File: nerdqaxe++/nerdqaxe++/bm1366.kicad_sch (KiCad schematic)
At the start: 82 parts, among them U19 BM1370_mode1, U20 BM1370, U25 BM1370_mode1, U26 BM1370_mode1, U6 SN74AVC4T774, U8 25MHz

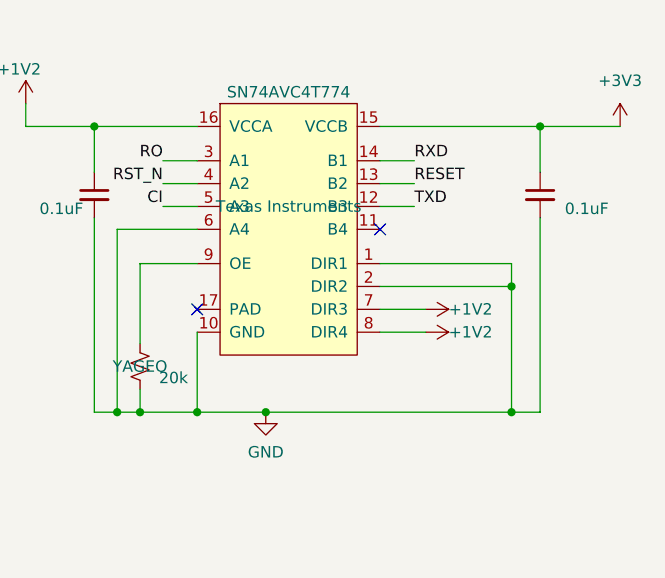
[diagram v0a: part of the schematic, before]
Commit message: Rev. 6.1
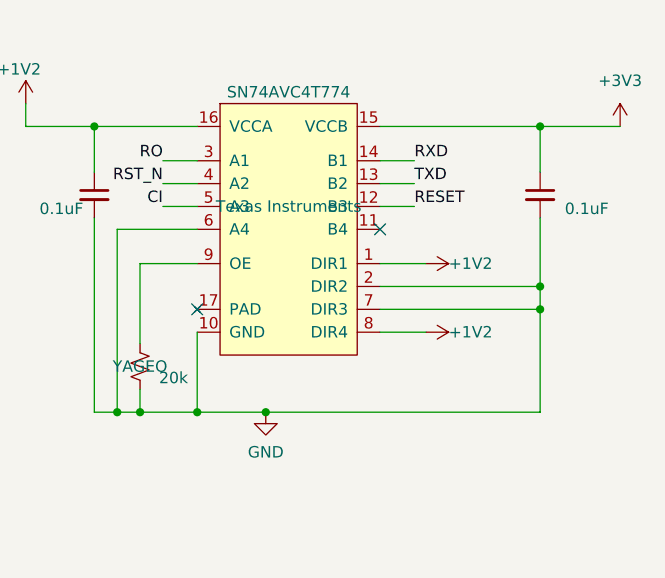
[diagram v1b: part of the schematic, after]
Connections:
- net +1V2: now also U6.1 (DIR1); no longer U6.7 (DIR3)
- net GND: now also U6.7 (DIR3); no longer U6.1 (DIR1)
- net RESET: now also U6.12 (B3); no longer U6.13 (B2)
- net TXD: now also U6.13 (B2); no longer U6.12 (B3)
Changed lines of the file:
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@@
 	)
 	(junction
-		(at 376.555 157.48)
-		(diameter 0)
-		(color 0 0 0 0)
-	)
-	(junction
 		(at 209.55 257.81)
 		(diameter 0)
@@
 	)
 	(junction
-		(at 198.12 233.68)
+		(at 379.73 143.51)
 		(diameter 0)
 		(color 0 0 0 0)
 	)
 	(junction
-		(at 200.66 229.87)
+		(at 198.12 233.68)
 		(diameter 0)
 		(color 0 0 0 0)
 	)
 	(junction
-		(at 196.85 257.81)
+		(at 200.66 229.87)
 		(diameter 0)
 		(color 0 0 0 0)
 	)
 	(junction
-		(at 376.555 143.51)
+		(at 196.85 257.81)
 		(diameter 0)
 		(color 0 0 0 0)
@@
 	)
 	(junction
+		(at 379.73 146.05)
+		(diameter 0)
+		(color 0 0 0 0)
+	)
+	(junction
 		(at 156.21 81.28)
 		(diameter 0)
@@
 	(wire
 		(pts
-			(xy 361.95 140.97) (xy 376.555 140.97)
-		)
-		(stroke
-			(width 0)
-			(type default)
-		)
-	)
-	(wire
-		(pts
 			(xy 151.13 127) (xy 156.21 127)
 		)
@@
 	(wire
 		(pts
-			(xy 376.555 140.97) (xy 376.555 143.51)
-		)
-		(stroke
-			(width 0)
-			(type default)
-		)
-	)
-	(wire
-		(pts
 			(xy 220.98 250.19) (xy 220.98 248.92)
 		)
@@
 	(wire
 		(pts
-			(xy 376.555 143.51) (xy 376.555 157.48)
-		)
-		(stroke
-			(width 0)
-			(type default)
-		)
-	)
-	(wire
-		(pts
 			(xy 179.07 55.88) (xy 179.07 41.91)
 		)
@@
 	(wire
 		(pts
+			(xy 349.25 157.48) (xy 379.73 157.48)
+		)
+		(stroke
+			(width 0)
+			(type default)
+		)
+	)
+	(wire
+		(pts
 			(xy 262.89 81.28) (xy 262.89 83.82)
 		)
@@
 	(wire
 		(pts
-			(xy 361.95 146.05) (xy 367.03 146.05)
-		)
-		(stroke
-			(width 0)
-			(type default)
-		)
-	)
-	(wire
-		(pts
 			(xy 118.11 161.29) (xy 102.87 161.29)
 		)
@@
 	(wire
 		(pts
-			(xy 361.95 143.51) (xy 376.555 143.51)
-		)
-		(stroke
-			(width 0)
-			(type default)
-		)
-	)
-	(wire
-		(pts
 			(xy 29.21 31.75) (xy 38.1 31.75)
 		)
@@
 	(wire
 		(pts
+			(xy 361.95 143.51) (xy 379.73 143.51)
+		)
+		(stroke
+			(width 0)
+			(type default)
+		)
+	)
+	(wire
+		(pts
 			(xy 156.21 135.89) (xy 198.12 135.89)
 		)
@@
 	(wire
 		(pts
+			(xy 361.95 140.97) (xy 367.03 140.97)
+		)
+		(stroke
+			(width 0)
+			(type default)
+		)
+	)
+	(wire
+		(pts
 			(xy 187.96 255.27) (xy 187.96 257.81)
 		)
@@
 	(wire
 		(pts
+			(xy 379.73 146.05) (xy 379.73 157.48)
+		)
+		(stroke
+			(width 0)
+			(type default)
+		)
+	)
+	(wire
+		(pts
 			(xy 191.77 227.33) (xy 191.77 229.87)
 		)
@@
 	(wire
 		(pts
-			(xy 379.73 135.89) (xy 379.73 157.48)
+			(xy 379.73 135.89) (xy 379.73 143.51)
 		)
 		(stroke
@@
 	(wire
 		(pts
+			(xy 379.73 143.51) (xy 379.73 146.05)
+		)
+		(stroke
+			(width 0)
+			(type default)
+		)
+	)
+	(wire
+		(pts
 			(xy 167.64 53.34) (xy 199.39 53.34)
 		)
@@
 	(wire
 		(pts
-			(xy 349.25 157.48) (xy 376.555 157.48)
+			(xy 135.89 39.37) (xy 135.89 41.91)
 		)
 		(stroke
@@
 	(wire
 		(pts
-			(xy 135.89 39.37) (xy 135.89 41.91)
+			(xy 260.35 41.91) (xy 262.89 41.91)
 		)
 		(stroke
@@
 	(wire
 		(pts
-			(xy 260.35 41.91) (xy 262.89 41.91)
+			(xy 207.01 242.57) (xy 210.82 242.57)
 		)
 		(stroke
@@
 	(wire
 		(pts
-			(xy 207.01 242.57) (xy 210.82 242.57)
+			(xy 104.14 198.12) (xy 104.14 199.39)
 		)
 		(stroke
@@
 	(wire
 		(pts
-			(xy 104.14 198.12) (xy 104.14 199.39)
+			(xy 102.87 76.2) (xy 118.11 76.2)
 		)
 		(stroke
@@
 	(wire
 		(pts
-			(xy 102.87 76.2) (xy 118.11 76.2)
+			(xy 361.95 146.05) (xy 379.73 146.05)
 		)
 		(stroke
@@
 	(wire
 		(pts
-			(xy 376.555 157.48) (xy 379.73 157.48)
-		)
-		(stroke
-			(width 0)
-			(type default)
-		)
-	)
-	(wire
-		(pts
 			(xy 198.12 58.42) (xy 198.12 81.28)
 		)
@@
 		)
 	)
-	(label "RESET"
-		(at 365.76 132.08 0)
-		(effects
-			(font
-				(size 1.27 1.27)
-			)
-			(justify left bottom)
-		)
-	)
 	(label "CI"
 		(at 337.82 134.62 180)
@@
 		)
 	)
-	(label "TXD"
-		(at 365.76 134.62 0)
-		(effects
-			(font
-				(size 1.27 1.27)
-			)
-			(justify left bottom)
-		)
-	)
 	(label "RXD"
 		(at 365.76 129.54 0)
@@
 		)
 	)
+	(label "TXD"
+		(at 365.76 132.08 0)
+		(effects
+			(font
+				(size 1.27 1.27)
+			)
+			(justify left bottom)
+		)
+	)
 	(label "RST_N"
 		(at 101.6 60.96 0)
@@
 		)
 	)
+	(label "RESET"
+		(at 365.76 134.62 0)
+		(effects
+			(font
+				(size 1.27 1.27)
+			)
+			(justify left bottom)
+		)
+	)
 	(label "RO"
 		(at 337.82 129.54 180)
@@
 	(symbol
 		(lib_id "power:+1V2")
-		(at 367.03 146.05 270)
+		(at 367.03 140.97 270)
 		(unit 1)
 		(exclude_from_sim no)
@@
 		(dnp no)
 		(property "Reference" "#PWR0177"
-			(at 363.22 146.05 0)
+			(at 363.22 140.97 0)
 			(effects
 				(font
@@
 		)
 		(property "Value" "+1V2"
-			(at 369.57 146.05 90)
+			(at 369.57 140.97 90)
 			(effects
 				(font
@@
 		)
 		(property "Footprint" ""
-			(at 367.03 146.05 0)
+			(at 367.03 140.97 0)
 			(effects
 				(font
@@
 		)
 		(property "Datasheet" ""
-			(at 367.03 146.05 0)
+			(at 367.03 140.97 0)
 			(effects
 				(font
@@
 		)
 		(property "Description" "Power symbol creates a global label with name \"+1V2\""
-			(at 367.03 146.05 0)
+			(at 367.03 140.97 0)
 			(effects
 				(font
